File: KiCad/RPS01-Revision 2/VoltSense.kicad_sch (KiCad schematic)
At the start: 12 parts, among them U13 UA741CDT, U15 UA741CDT

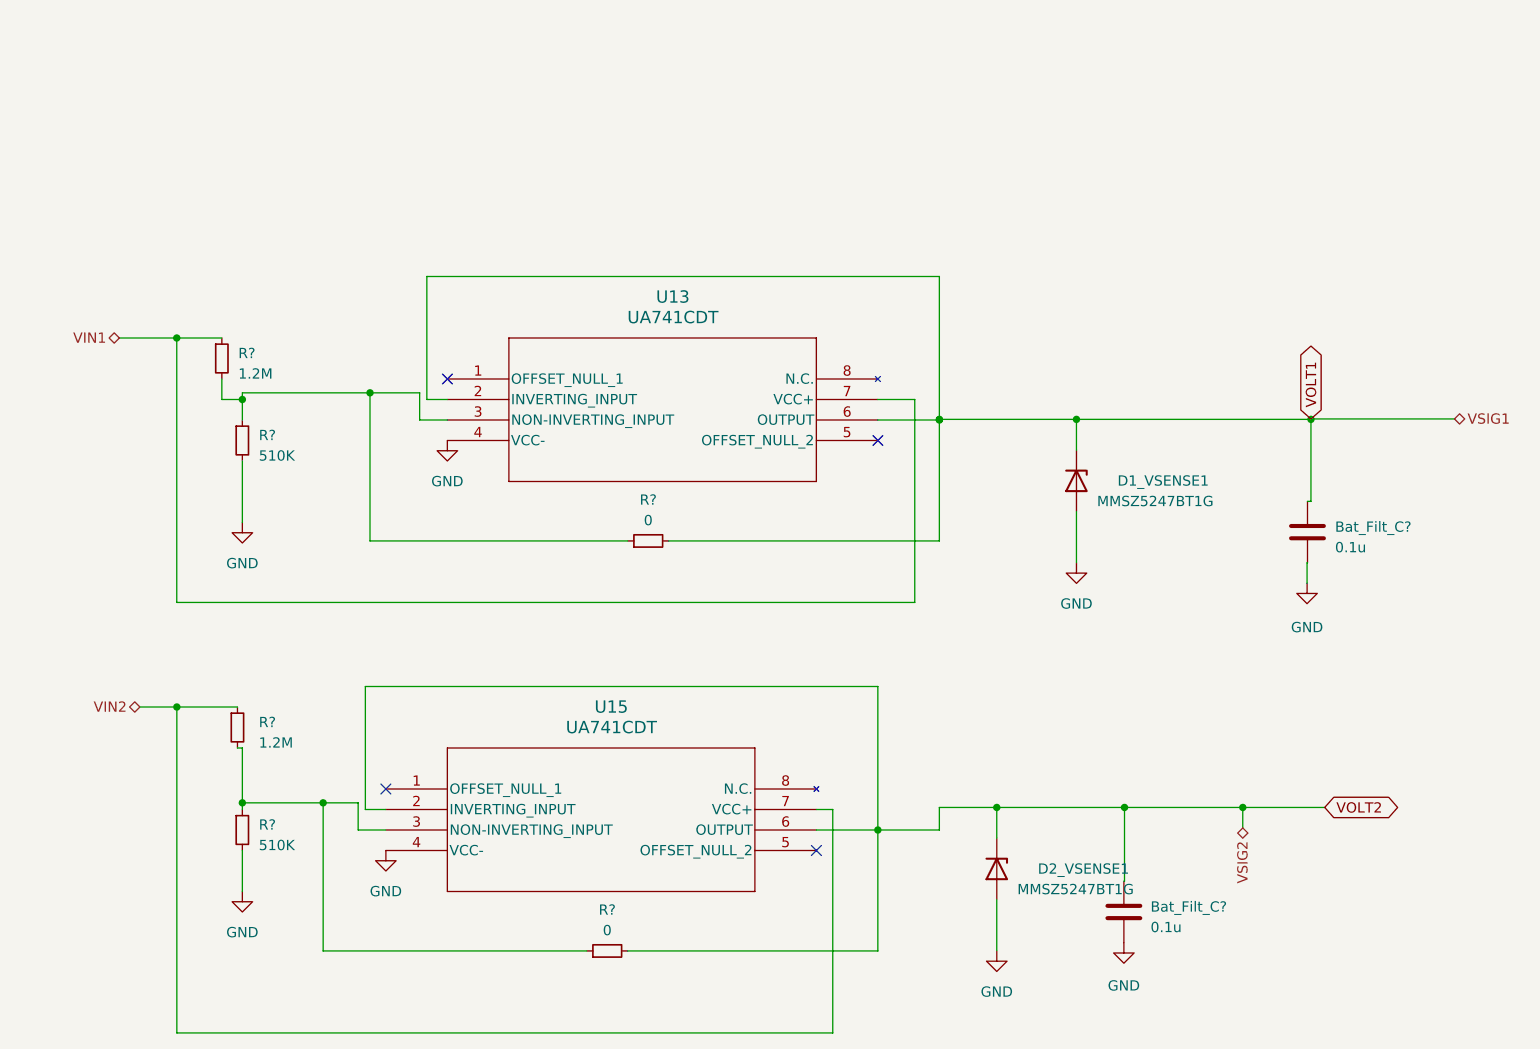
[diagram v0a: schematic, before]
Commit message: updates
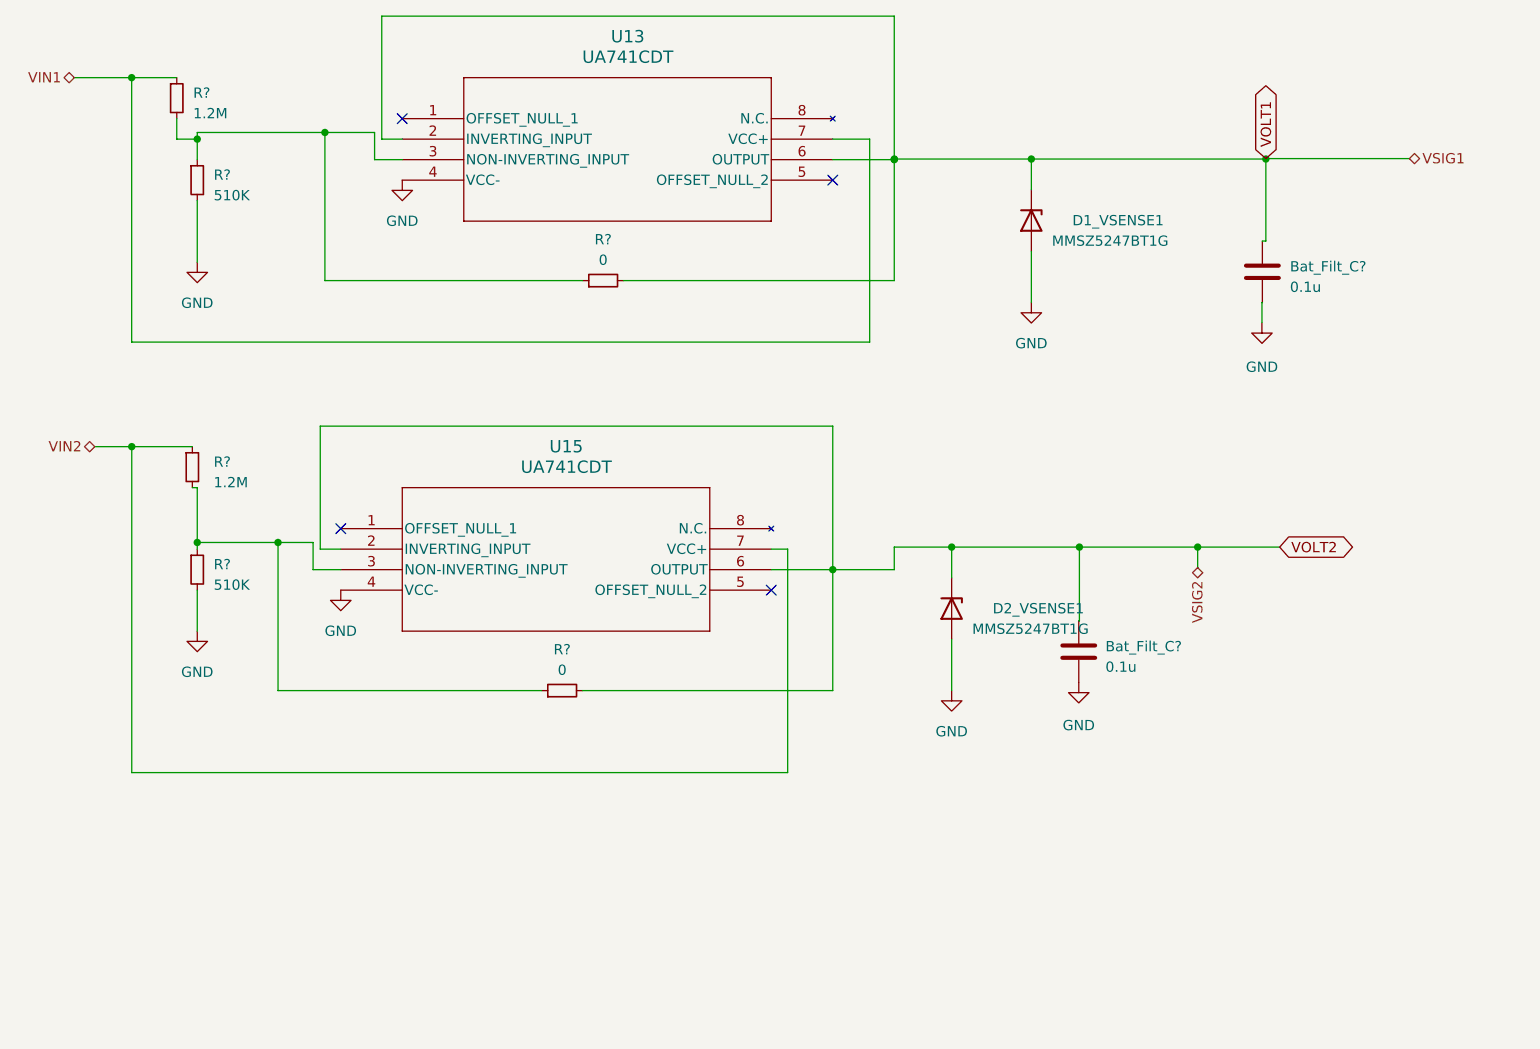
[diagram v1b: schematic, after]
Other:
- moved on the sheet: Bat_Filt_C?, D1_VSENSE1, D2_VSENSE1, R?, U13, U15
